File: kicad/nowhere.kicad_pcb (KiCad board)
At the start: 2 copper layers, 80 x 69.8 mm, 27 parts, among them J1 DIN-4, J2 DIN-4, J3 DIN-4, J4 DIN-4, J5 DIN-4, J6 DIN-4, J7 DIN-4, J8 DIN-4, J9 Barrel_Jack, U1 Teensy3.6, U2 74HC245, U3 LM2576T-5

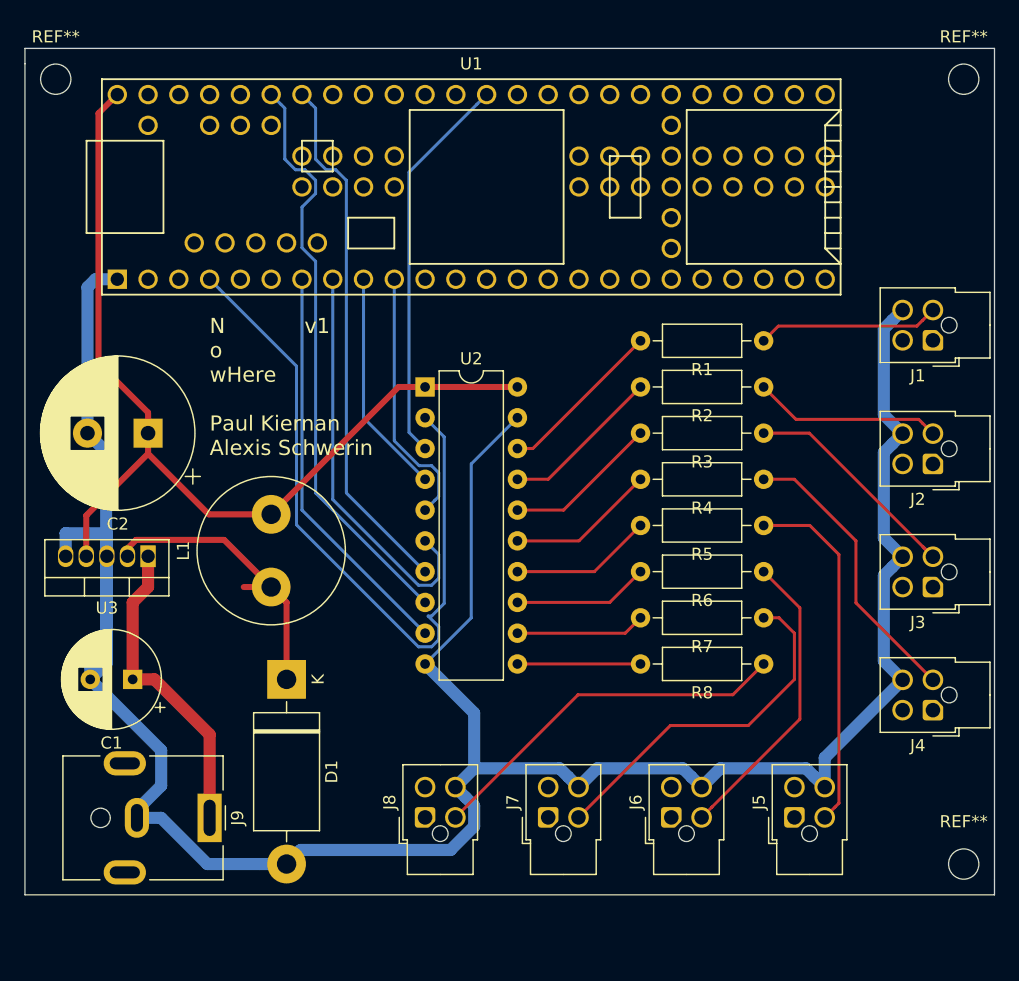
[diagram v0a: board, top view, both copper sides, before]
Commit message: PCB version 2
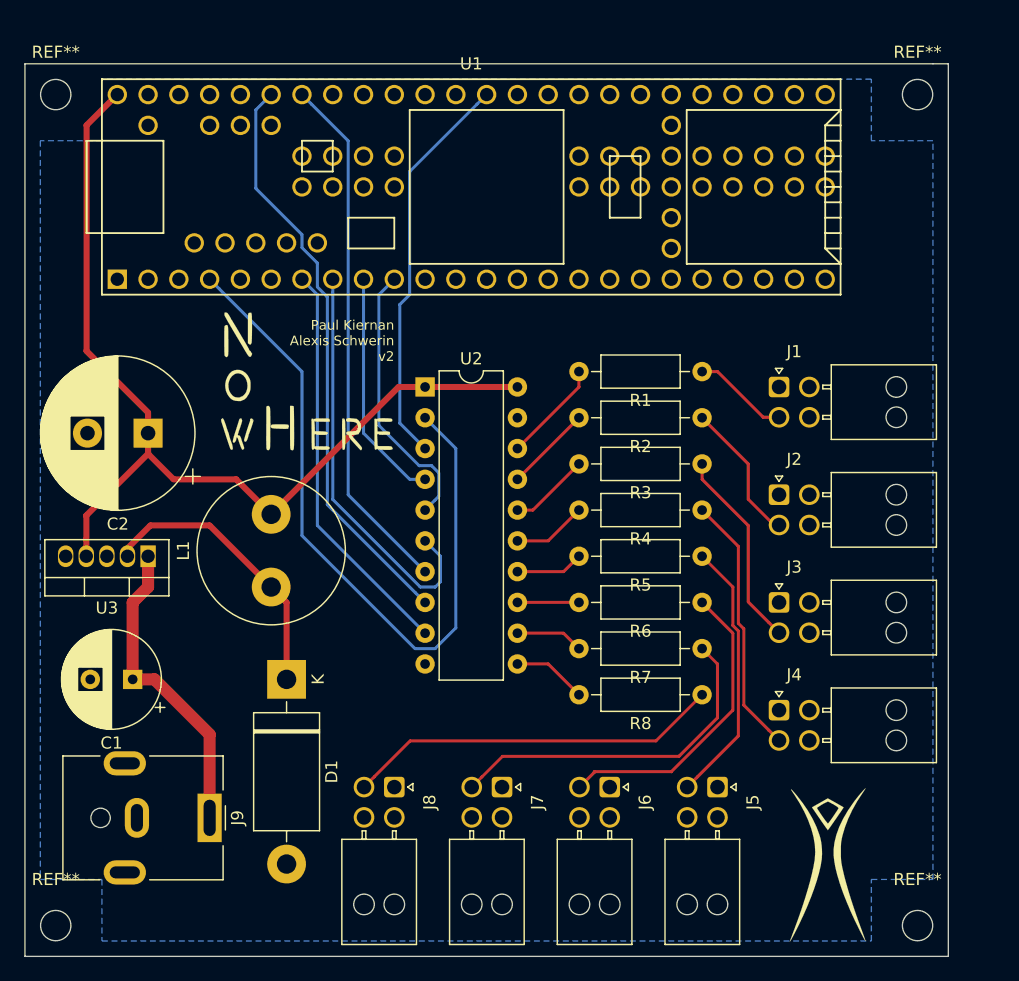
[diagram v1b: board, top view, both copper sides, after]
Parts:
- added G***: LOGO, nowhere:the-man-silkscreen, F.Cu at (129.5, 80.0)
- added G***: LOGO, nowhere:nowhere-silkscreen-small, F.Cu at (87.6, 39.4)
- added G***: LOGO, nowhere:nowhere-silkscreen, B.Cu at (120.7, 38.1)
- added G***: LOGO, nowhere:nowhere-silkscreen, B.Cu at (96.5, 49.5)
- added G***: LOGO, nowhere:nowhere-silkscreen, B.Cu at (114.3, 69.8)
- added G***: LOGO, nowhere:nowhere-silkscreen, B.Cu at (82.5, 63.5)
- added G***: LOGO, nowhere:nowhere-silkscreen, B.Cu at (87.6, 33.0)
- added REF**: MountingHole_2.5mm, MountingHole:MountingHole_2.5mm, F.Cu at (137.2, 85.1)
- J1, J2, J3, J4, J5, J6, J7, J8: footprint Connector_Molex:Molex_Nano-Fit_105310-xx04_2x02_P2.50mm_Vertical -> Connector_Molex:Molex_Nano-Fit_105314-xx04_2x02_P2.50mm_Horizontal
- moved REF** 75.1 mm to (66.0, 85.1)
- moved J1 13.3 mm to (125.7, 40.6), turned to 0 degrees
- moved J2 13.0 mm to (125.7, 49.5), turned to 0 degrees
- moved J3 12.8 mm to (125.7, 58.4), turned to 0 degrees
- moved J4 12.7 mm to (125.7, 67.3), turned to 0 degrees
- moved J5 6.82 mm to (120.7, 73.7), turned to 270 degrees
- moved R8 5.68 mm to (119.4, 66.0)
- moved R1 5.68 mm to (119.4, 39.4)
- moved R2 5.68 mm to (119.4, 43.2)
- moved R3 5.68 mm to (119.4, 47.0)
- moved R4 5.68 mm to (119.4, 50.8)
- moved R5 5.68 mm to (119.4, 54.6)
- moved R6 5.68 mm to (119.4, 58.4)
- moved R7 5.68 mm to (119.4, 62.2)
- moved J6 5.66 mm to (111.8, 73.7), turned to 270 degrees
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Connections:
- J1 pad 1: +12V -> Net-(J1-Pad1)
- J2 pad 1: +12V -> Net-(J2-Pad1)
- J3 pad 1: +12V -> Net-(J3-Pad1)
- J4 pad 1: +12V -> Net-(J4-Pad1)
- J5 pad 1: +12V -> Net-(J5-Pad1)
- J6 pad 1: +12V -> Net-(J6-Pad1)
- J7 pad 1: +12V -> Net-(J7-Pad1)
- J8 pad 1: +12V -> Net-(J8-Pad1)
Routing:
- net GND: track 217.4 -> 0.00 mm
- net data4_out: track 29.4 -> 22.0 mm
- net data0_out: track 15.0 -> 7.91 mm
- net Net-(R6-Pad2): track 11.2 -> 5.08 mm
- net Net-(R3-Pad2): track 12.8 -> 6.66 mm
- net Net-(R2-Pad2): track 13.3 -> 7.18 mm
- net Net-(R5-Pad2): track 11.7 -> 5.61 mm
- net Net-(R4-Pad2): track 12.3 -> 6.13 mm
- net Net-(R1-Pad2): track 13.8 -> 8.45 mm
- net Net-(R7-Pad2): track 10.7 -> 5.61 mm
- net Net-(R8-Pad2): track 10.2 -> 6.13 mm
- net data1_out: track 15.6 -> 11.7 mm
- net data2_out: track 19.4 -> 16.6 mm
- net data3_out: track 23.8 -> 21.6 mm
- net Net-(D1-Pad1): track 25.5 -> 24.2 mm
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- added copper zone on B.Cu, net GND
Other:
- board size 80 x 69.8 mm -> 76.2 x 73.7 mm
- board text added: "Paul Kiernan Alexis Schwerin v2"
- board text removed: "N v1 o wHere Paul Kiernan Alexis Schwerin"
